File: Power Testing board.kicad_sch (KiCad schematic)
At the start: 9 parts, among them J1 Conn_01x26_Pin, J2 Conn_01x26_Pin, J3 Conn_01x26_Pin, J4 Conn_01x26_Pin, U1 INA260, U2 INA260, U3 INA260, U4 INA260

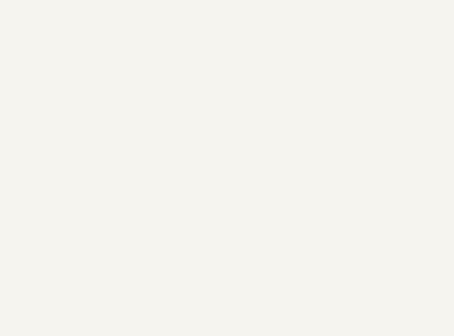
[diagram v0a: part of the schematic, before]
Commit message: testing res
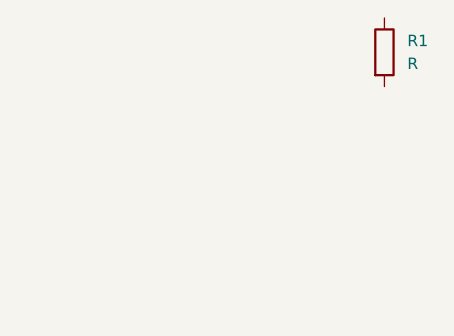
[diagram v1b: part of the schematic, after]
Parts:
- added R1: R, symbol Device:R
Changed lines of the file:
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@@
+	)
+	(symbol
+		(lib_id "Device:R")
+		(at 260.35 33.02 0)
+		(unit 1)
+		(body_style 1)
+		(exclude_from_sim no)
+		(in_bom yes)
+		(on_board yes)
+		(in_pos_files yes)
+		(dnp no)
+		(fields_autoplaced yes)
+		(property "Reference" "R1"
+			(at 262.89 31.7499 0)
+			(show_name no)
+			(do_not_autoplace no)
+			(effects
+				(font
+					(size 1.27 1.27)
+				)
+				(justify left)
+			)
+		)
+		(property "Value" "R"
+			(at 262.89 34.2899 0)
+			(show_name no)
+			(do_not_autoplace no)
+			(effects
+				(font
+					(size 1.27 1.27)
+				)
+				(justify left)
+			)
+		)
+		(property "Footprint" ""
+			(at 258.572 33.02 90)
+			(hide yes)
+			(show_name no)
+			(do_not_autoplace no)
+			(effects
+				(font
+					(size 1.27 1.27)
+				)
+			)
+		)
+		(property "Datasheet" ""
+			(at 260.35 33.02 0)
+			(hide yes)
+			(show_name no)
+			(do_not_autoplace no)
+			(effects
+				(font
+					(size 1.27 1.27)
+				)
+			)
+		)
+		(property "Description" "Resistor"
+			(at 260.35 33.02 0)
+			(hide yes)
+			(show_name no)
+			(do_not_autoplace no)
+			(effects
+				(font
+					(size 1.27 1.27)
+				)
+			)
+		)
+		(pin "1"
+		)
+		(pin "2"
+		)
+		(instances
+			(project "Power Testing board"
+				(path "/8dfe3f75-d63d-44af-a5fd-924c068dba42"
+					(reference "R1")
+					(unit 1)
+				)
+			)
+		)
 	)
 	(symbol

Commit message: test
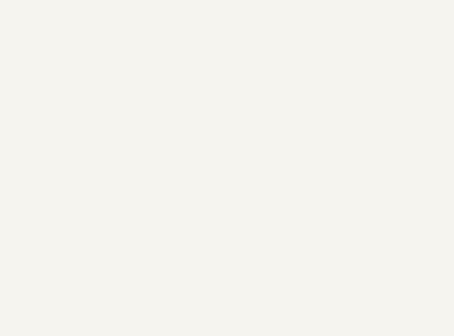
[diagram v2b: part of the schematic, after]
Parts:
- removed R1: R, symbol Device:R
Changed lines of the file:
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@@
-	)
-	(symbol
-		(lib_id "Device:R")
-		(at 260.35 33.02 0)
-		(unit 1)
-		(body_style 1)
-		(exclude_from_sim no)
-		(in_bom yes)
-		(on_board yes)
-		(in_pos_files yes)
-		(dnp no)
-		(fields_autoplaced yes)
-		(property "Reference" "R1"
-			(at 262.89 31.7499 0)
-			(show_name no)
-			(do_not_autoplace no)
-			(effects
-				(font
-					(size 1.27 1.27)
-				)
-				(justify left)
-			)
-		)
-		(property "Value" "R"
-			(at 262.89 34.2899 0)
-			(show_name no)
-			(do_not_autoplace no)
-			(effects
-				(font
-					(size 1.27 1.27)
-				)
-				(justify left)
-			)
-		)
-		(property "Footprint" ""
-			(at 258.572 33.02 90)
-			(hide yes)
-			(show_name no)
-			(do_not_autoplace no)
-			(effects
-				(font
-					(size 1.27 1.27)
-				)
-			)
-		)
-		(property "Datasheet" ""
-			(at 260.35 33.02 0)
-			(hide yes)
-			(show_name no)
-			(do_not_autoplace no)
-			(effects
-				(font
-					(size 1.27 1.27)
-				)
-			)
-		)
-		(property "Description" "Resistor"
-			(at 260.35 33.02 0)
-			(hide yes)
-			(show_name no)
-			(do_not_autoplace no)
-			(effects
-				(font
-					(size 1.27 1.27)
-				)
-			)
-		)
-		(pin "1"
-		)
-		(pin "2"
-		)
-		(instances
-			(project "Power Testing board"
-				(path "/8dfe3f75-d63d-44af-a5fd-924c068dba42"
-					(reference "R1")
-					(unit 1)
-				)
-			)
-		)
 	)
 	(symbol
